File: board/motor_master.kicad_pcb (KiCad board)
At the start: 2 copper layers, 42 x 52 mm, 38 parts, among them IC1 LM1117MPX-3.3_NOPB, IC2 SN65HVD232DR, J1 PWR, J2 USB4105-GF-A, J3 FTDI, J4 CAN, J5 TERM, J6 PWM1, J7 PWM2, U1 ESP32-S3-WROOM-1-N8

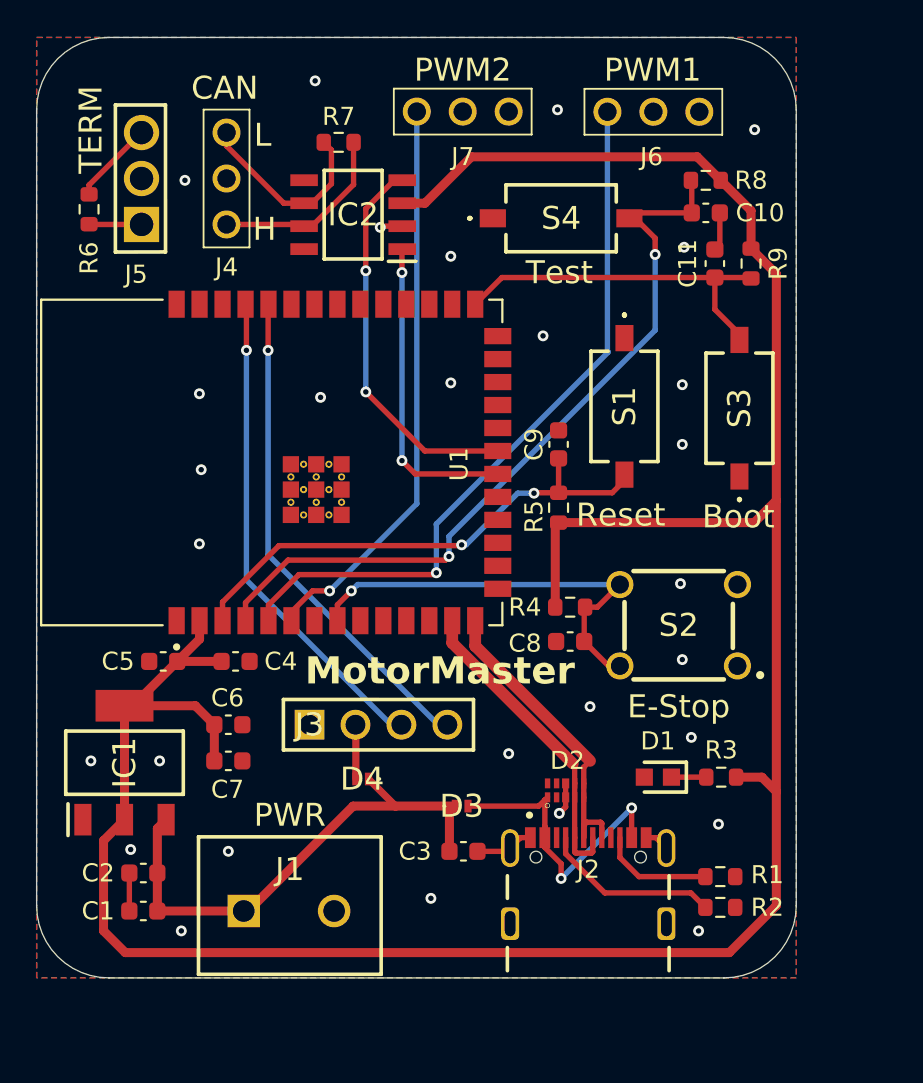
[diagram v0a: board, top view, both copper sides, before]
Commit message: Board revisions from design review
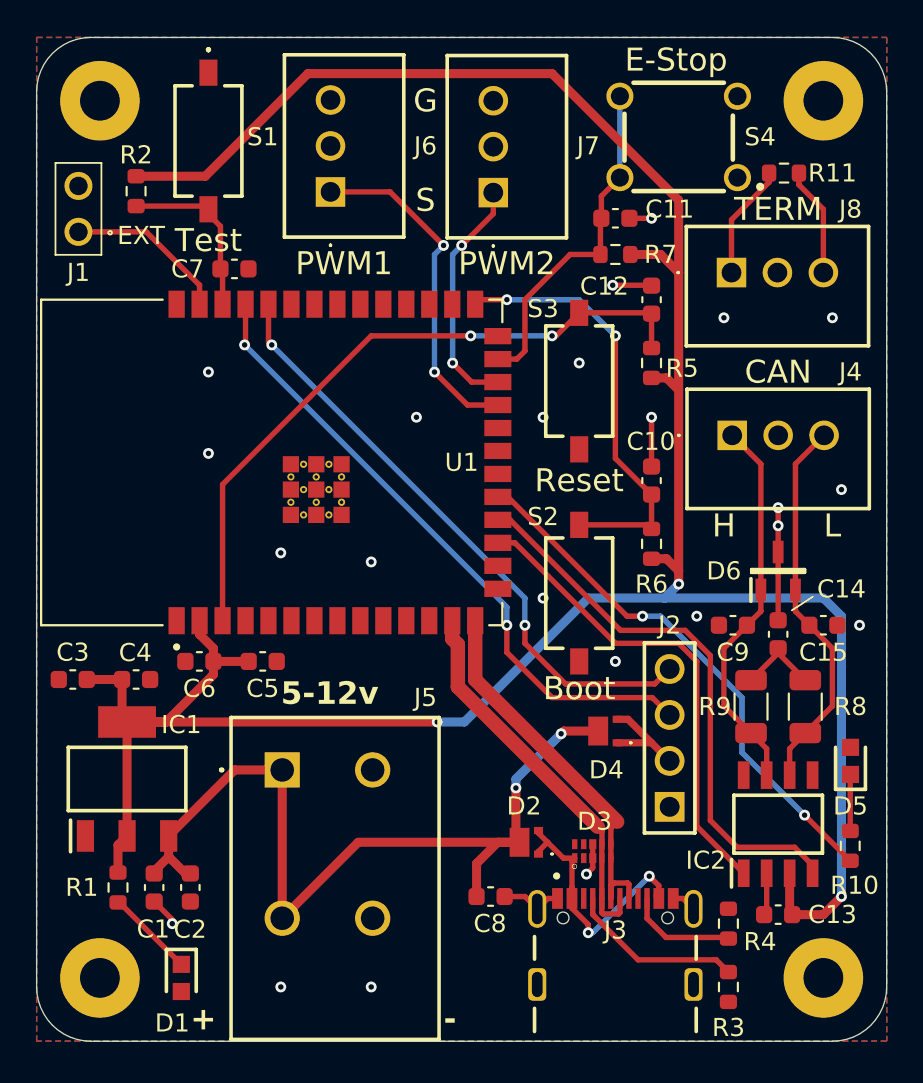
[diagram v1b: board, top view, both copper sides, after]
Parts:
- added C13: 0.1uF, Capacitor_SMD:C_0603_1608Metric, F.Cu at (167.5, 122.0)
- added C14: 4.7n, Capacitor_SMD:C_0603_1608Metric, F.Cu at (167.5, 106.5)
- added C15: 100p, Capacitor_SMD:C_0603_1608Metric, F.Cu at (170.0, 106.0)
- added C9: 100p, Capacitor_SMD:C_0603_1608Metric, F.Cu at (165.0, 106.0)
- added D5: 150060RS75000, SamacSys_Parts:LEDC1608X80N, F.Cu at (171.5, 113.5)
- added D6: SZNUP2105LT1G, SamacSys_Parts:SOT96P237X111-3N, F.Cu at (167.5, 103.0)
- added J1: EXT, SamacSys_Parts:TSW-102-XX-YY-S, F.Cu at (128.8, 84.2)
- added R10: 47, Resistor_SMD:R_0603_1608Metric, F.Cu at (171.5, 118.2)
- added R2: 10k, Resistor_SMD:R_0603_1608Metric, F.Cu at (132.0, 82.0)
- added REF**: MountingHole_2.2mm_M2_Pad, MountingHole:MountingHole_2.2mm_M2_Pad, F.Cu at (170.0, 77.0)
- added REF**: MountingHole_2.2mm_M2_Pad, MountingHole:MountingHole_2.2mm_M2_Pad, F.Cu at (130.0, 125.5)
- added REF**: MountingHole_2.2mm_M2_Pad, MountingHole:MountingHole_2.2mm_M2_Pad, F.Cu at (130.0, 77.0)
- added REF**: MountingHole_2.2mm_M2_Pad, MountingHole:MountingHole_2.2mm_M2_Pad, F.Cu at (170.0, 125.5)
- D2: renamed from D3; value D5V0S1U2LP-7B -> PTVS18VU1UPAZ; footprint SamacSys_Parts:D5V0S1U2LP7B -> SamacSys_Parts:PMEG6020EPA115
- D4: value D5V0S1U2LP-7B -> PTVS18VU1UPAZ; footprint SamacSys_Parts:D5V0S1U2LP7B -> SamacSys_Parts:PMEG6020EPA115
- J4, J6, J7: footprint SamacSys_Parts:TSW-103-XX-YY-S -> SamacSys_Parts:1719710103
- J5: renamed from J1; value PWR -> 5-12V; footprint SamacSys_Parts:SHDR2W70P0X500_1X2_1000X750X1160P -> SamacSys_Parts:1190297
- J8: renamed from J5; footprint SamacSys_Parts:RHDR3W79P0X254_1X3_813X241X851P -> SamacSys_Parts:1719710103
- R1: renamed from R3; value 5.1k -> 47
- R8: value 10k -> 60; footprint Resistor_SMD:R_0603_1608Metric -> Resistor_SMD:R_1206_3216Metric
- R9: renamed from R7; value 120 -> 60; footprint Resistor_SMD:R_0603_1608Metric -> Resistor_SMD:R_1206_3216Metric
- moved IC2 41.1 mm to (167.5, 117.0), turned to 90 degrees
- moved R9 38.6 mm to (166.0, 110.5), turned to -90 degrees
- moved R11 38.5 mm to (167.8, 81.0), turned to 180 degrees
- moved R1 33.9 mm to (131.0, 120.5), turned to 90 degrees
- moved J8 32.7 mm to (164.9, 86.5), turned to 180 degrees
- moved J4 30.3 mm to (165.0, 95.5), turned to 180 degrees
- moved R8 29.6 mm to (169.0, 110.5), turned to -90 degrees
- moved D1 28.6 mm to (134.5, 125.5), turned to -90 degrees
- moved S4 27.0 mm to (162.0, 79.0)
- moved C7 26.2 mm to (137.4, 86.3)
- moved C11 23.5 mm to (158.5, 83.5), turned to 180 degrees
- moved J2 20.4 mm to (161.5, 116.0), turned to 90 degrees
- moved S1 20.0 mm to (136.0, 79.2), turned to -90 degrees
- moved R7 19.7 mm to (158.5, 85.5), turned to 0 degrees
- moved R6 16.4 mm to (160.5, 101.5), turned to -90 degrees
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- renumbered C2 to C1, C11 to C10, C8 to C11, C9 to C12, C1 to C2, C7 to C3, C6 to C4, C4 to C5, C5 to C6, C10 to C7, C3 to C8, D2 to D3, J3 to J2, J2 to J3, R6 to R11, R2 to R3, R1 to R4, R9 to R6, R4 to R7, S4 to S1, S3 to S2, S1 to S3, S2 to S4
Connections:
- C11 pad 2: GPIO15 -> GPIO48
- C7 pad 2: GPIO4 -> GPIO2
- D2 pad 1: VCC_IN -> Net-(D2-A_1)
- D2 pad 2: Net-(D2-IO1) -> Net-(D2-A_1)
- D3 pad 1: Net-(D2-IO1) -> Net-(D2-A_1)
- D4 pad 1: VCC_IN -> Net-(D4-A_1)
- D4 pad 2: Net-(D4-A) -> Net-(D4-A_1)
- IC2 pad 1: GPIO12 -> GPIO9
- IC2 pad 4: GPIO13 -> GPIO10
- IC2 pad 6: Net-(IC2-CANL) -> Net-(D6-CANL)
- J2 pad 2: Net-(D4-A) -> Net-(D4-A_1)
- J3 pad A4_B9: Net-(D2-IO1) -> Net-(D2-A_1)
- J3 pad B4_A9: Net-(D2-IO1) -> Net-(D2-A_1)
- J4 pad 2: unconnected-(J4-NC-Pad2) -> GND
- J4 pad 3: Net-(IC2-CANL) -> Net-(D6-CANL)
- J5 pad 2: GND -> VCC_IN
- J6 pad 1: GPIO5 -> GPIO21
- J7 pad 1: GPIO6 -> GPIO47
- J8 pad 2: unconnected-(J5-NC-Pad2) -> GND
- R7 pad 1: GPIO15 -> GPIO48
- R8 pad 1: GPIO4 -> Net-(C14-Pad2)
- R8 pad 2: VCC_3V3 -> Net-(D6-CANL)
- R9 pad 1: Net-(IC2-CANL) -> Net-(C14-Pad2)
- S1 pad 2: GPIO4 -> GPIO2
- S4 pad 2: GPIO15 -> GPIO48
- S4 pad 4: GPIO15 -> GPIO48
- U1 pad 17: unconnected-(U1-IO9-Pad17) -> GPIO9
- U1 pad 18: unconnected-(U1-IO10-Pad18) -> GPIO10
- U1 pad 19: unconnected-(U1-IO11-Pad19) -> GPIO11
- U1 pad 20: GPIO12 -> unconnected-(U1-IO12-Pad20)
- U1 pad 21: GPIO13 -> unconnected-(U1-IO13-Pad21)
- U1 pad 23: unconnected-(U1-IO21-Pad23) -> GPIO21
- U1 pad 24: unconnected-(U1-IO47-Pad24) -> GPIO47
- U1 pad 25: unconnected-(U1-IO48-Pad25) -> GPIO48
- U1 pad 38: unconnected-(U1-IO2-Pad38) -> GPIO2
- U1 pad 39: unconnected-(U1-IO1-Pad39) -> GPIO1
- U1 pad 4: GPIO4 -> unconnected-(U1-IO4-Pad4)
- U1 pad 5: GPIO5 -> unconnected-(U1-IO5-Pad5)
- U1 pad 6: GPIO6 -> unconnected-(U1-IO6-Pad6)
- U1 pad 8: GPIO15 -> unconnected-(U1-IO15-Pad8)
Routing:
- net GPIO4: track 42.3 -> 0.00 mm, vias 2 -> 0
- net GPIO5: track 40.3 -> 0.00 mm, vias 1 -> 0
- net GPIO6: track 31.6 -> 0.00 mm, vias 1 -> 0
- net GPIO10: track 0.00 -> 31.1 mm
- net GPIO11: track 0.00 -> 29.6 mm, vias 0 -> 2
- net GPIO9: track 0.00 -> 26.5 mm
- net GPIO15: track 23.9 -> 0.00 mm, vias 1 -> 0
- net GPIO13: track 21.4 -> 0.00 mm, vias 2 -> 0
- net Net-(D6-CANL): track 0.00 -> 21.3 mm
- net VCC_IN: track 28.9 -> 48.8 mm, vias 0 -> 2
- net GPIO21: track 0.00 -> 18.9 mm, vias 0 -> 2
- net GPIO48: track 0.00 -> 18.9 mm
- net GPIO12: track 17.3 -> 0.00 mm, vias 2 -> 0
- net Net-(D2-IO1): track 17.1 -> 0.00 mm, vias 2 -> 0
- net Net-(D2-A_1): track 0.00 -> 15.1 mm, vias 0 -> 2
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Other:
- board size 42 x 52 mm -> 47 x 55.5 mm
- rule pad_to_mask_clearance: 0.038 -> 0.0508
- board text added: "+"
- board text added: "-"
- board text added: "47x55.5mm"
- board text added: "5-12v"
- board text added: "G"
- board text added: "Robotics Academy 2024 v1"
- board text added: "S"
